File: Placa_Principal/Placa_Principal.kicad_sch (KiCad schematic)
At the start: 2 parts, among them U2 ESP32-S3-DevKitC

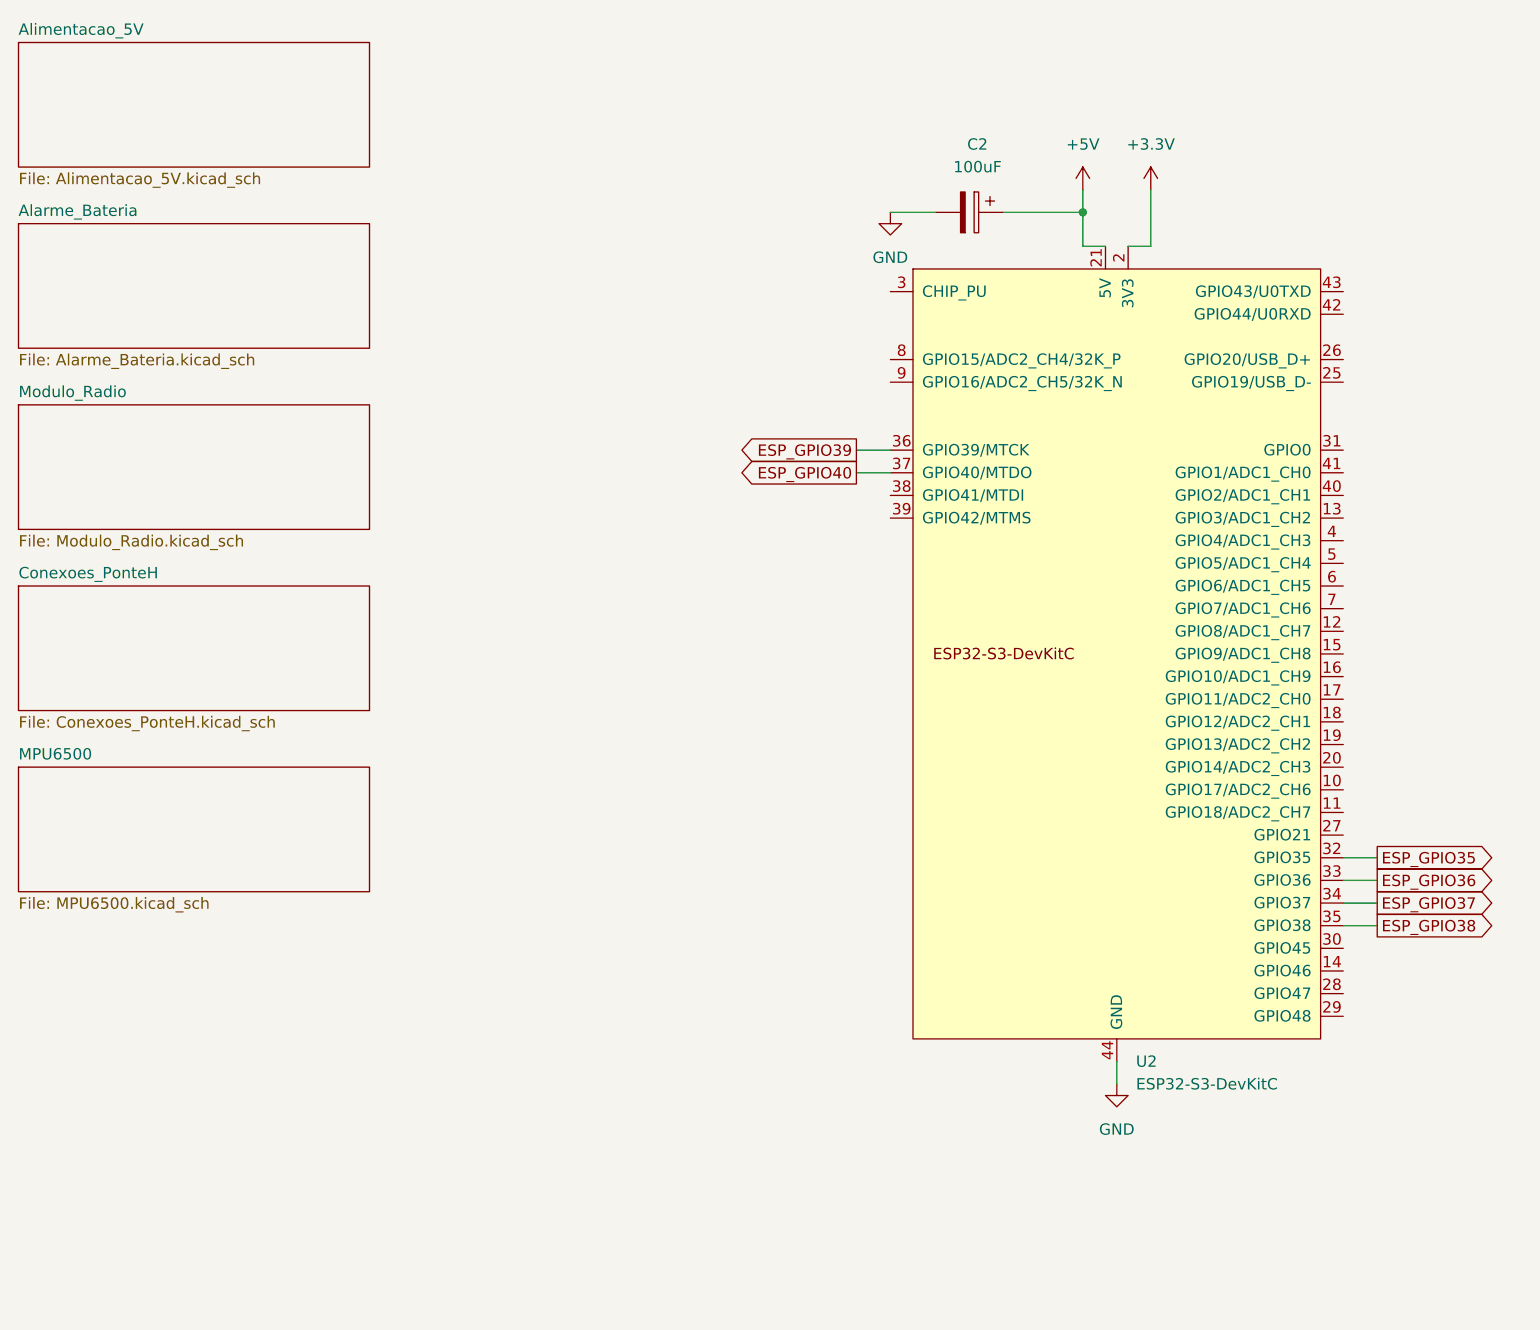
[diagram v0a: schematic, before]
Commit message: Segundo commit
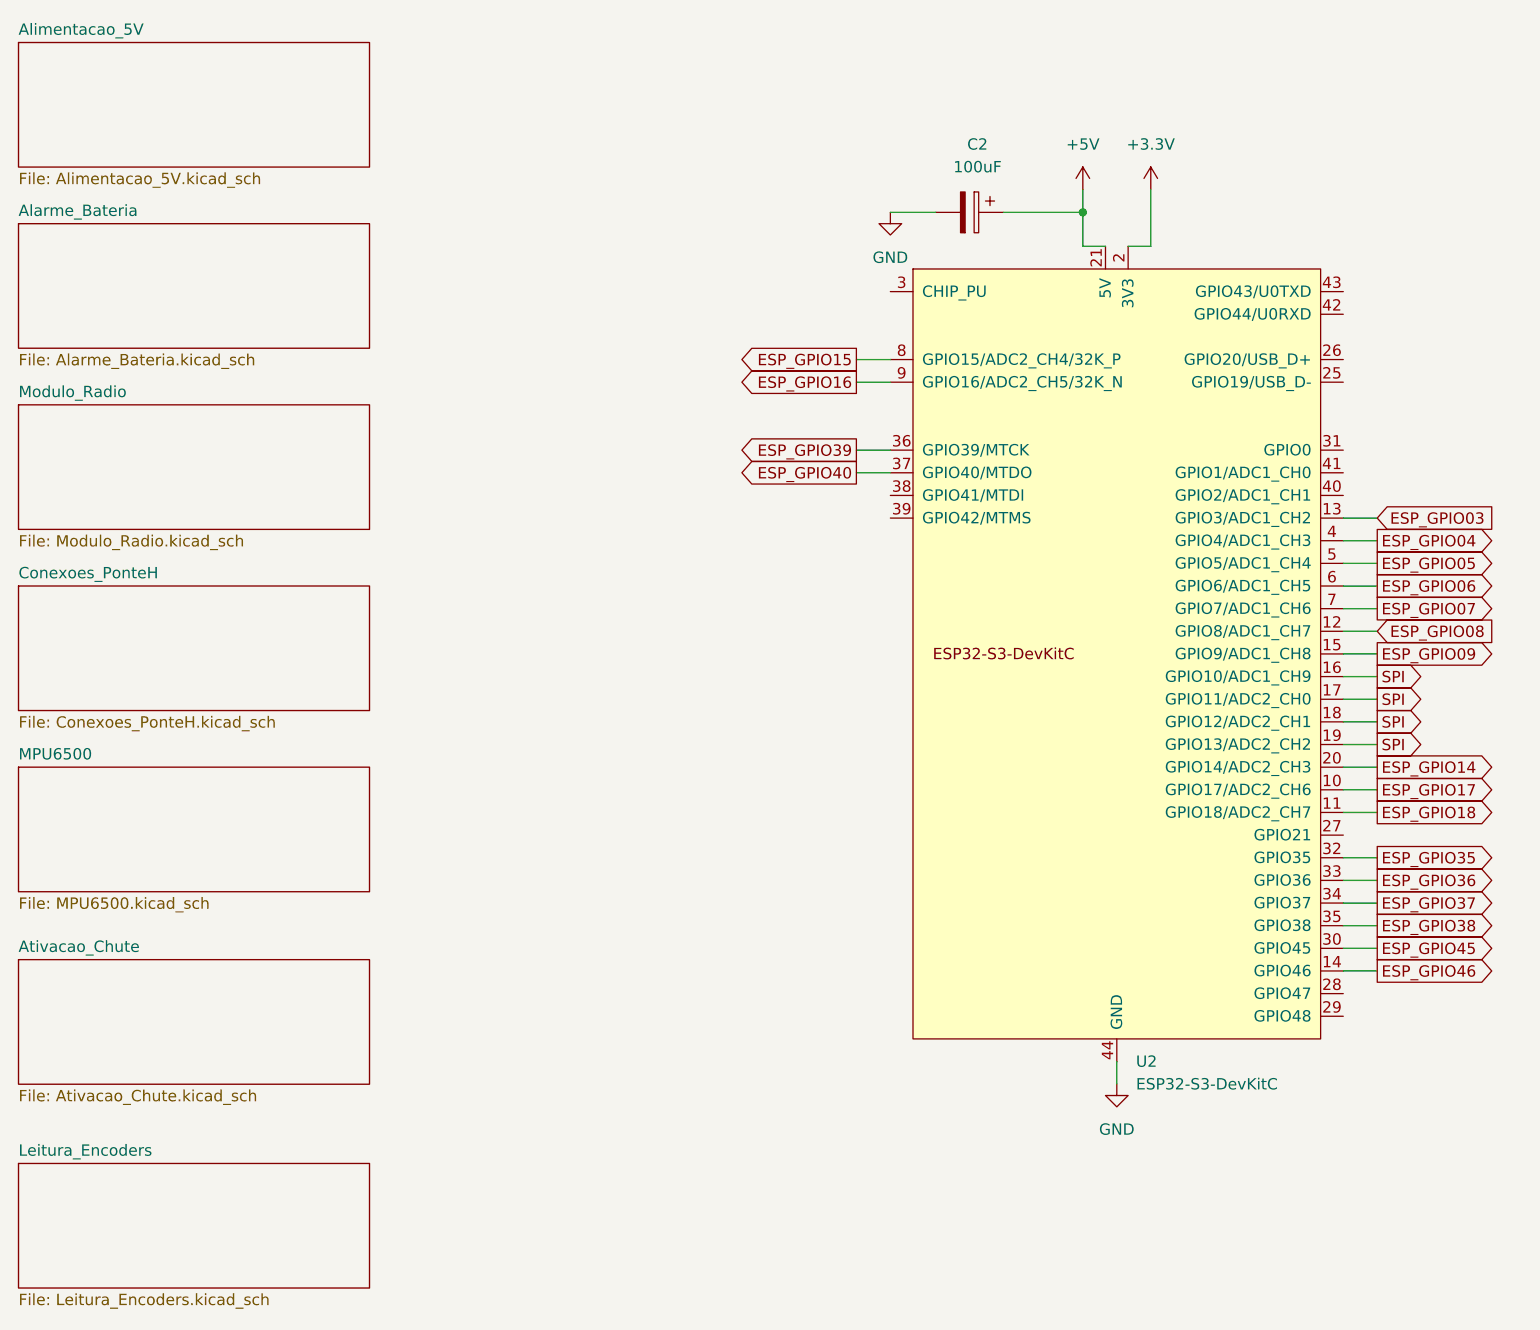
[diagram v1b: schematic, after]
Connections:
- net ESP_GPIO17: now reaches U2.10 (GPIO17/ADC2_CH6)
- net ESP_GPIO18: now reaches U2.11 (GPIO18/ADC2_CH7)
- net ESP_GPIO08: now reaches U2.12 (GPIO8/ADC1_CH7)
- net ESP_GPIO03: now reaches U2.13 (GPIO3/ADC1_CH2)
- net ESP_GPIO46: now reaches U2.14 (GPIO46)
- net ESP_GPIO09: now reaches U2.15 (GPIO9/ADC1_CH8)
- net SPI: now reaches U2.16 (GPIO10/ADC1_CH9)
- net SPI: now also U2.17 (GPIO11/ADC2_CH0), U2.18 (GPIO12/ADC2_CH1), U2.19 (GPIO13/ADC2_CH2)
- net ESP_GPIO14: now reaches U2.20 (GPIO14/ADC2_CH3)
- net ESP_GPIO45: now reaches U2.30 (GPIO45)
- net ESP_GPIO04: now reaches U2.4 (GPIO4/ADC1_CH3)
- net ESP_GPIO05: now reaches U2.5 (GPIO5/ADC1_CH4)
- net ESP_GPIO06: now reaches U2.6 (GPIO6/ADC1_CH5)
- net ESP_GPIO07: now reaches U2.7 (GPIO7/ADC1_CH6)
- net ESP_GPIO15: now reaches U2.8 (GPIO15/ADC2_CH4/32K_P)
- net ESP_GPIO16: now reaches U2.9 (GPIO16/ADC2_CH5/32K_N)
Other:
- added sheet Ativacao_Chute (Ativacao_Chute.kicad_sch)
- added sheet Leitura_Encoders (Leitura_Encoders.kicad_sch)
